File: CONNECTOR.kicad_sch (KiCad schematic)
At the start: 12 parts, among them J10 SWD, J17 SW_UART, J2 STM_IO, J7 CONNECTOR

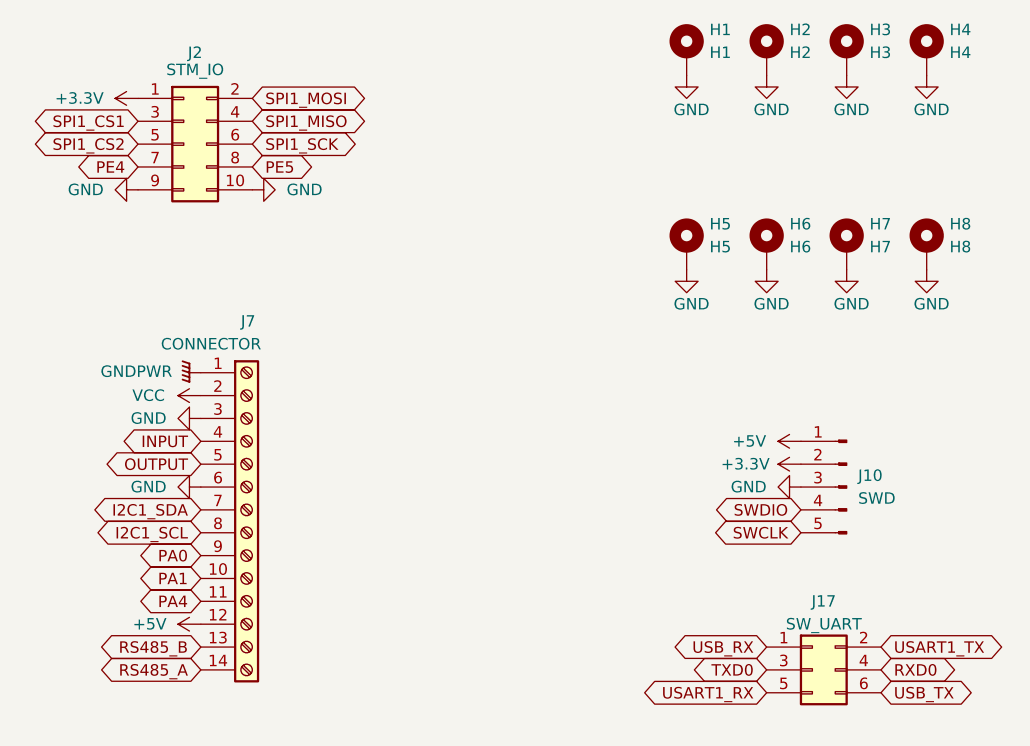
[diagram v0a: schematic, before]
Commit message: Add files via upload
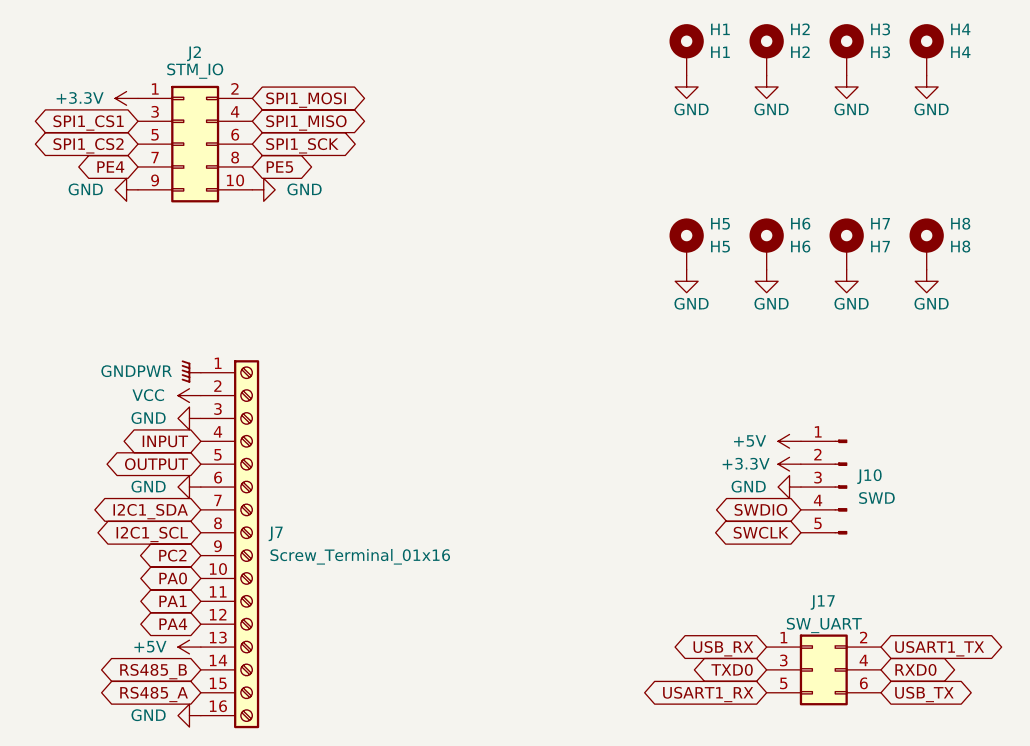
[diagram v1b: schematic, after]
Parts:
- removed J7: CONNECTOR, TerminalBlock_Phoenix:TerminalBlock_Phoenix_MKDS-1,5-14-5.08_1x14_P5.08mm_Horizontal, symbol Connector:Screw_Terminal_01x14
- added J7: Screw_Terminal_01x16, TerminalBlock_Phoenix:TerminalBlock_Phoenix_MKDS-1,5-16-5.08_1x16_P5.08mm_Horizontal, symbol Connector:Screw_Terminal_01x16
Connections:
- net +5V: now also J7.13 (Pin_13)
- net GND: now also J7.16 (Pin_16), J7.3 (Pin_3), J7.6 (Pin_6)
- net GNDPWR: now also J7.1 (Pin_1)
- net I2C1_SCL: now also J7.8 (Pin_8)
- net I2C1_SDA: now also J7.7 (Pin_7)
- net INPUT: now also J7.4 (Pin_4)
- net OUTPUT: now also J7.5 (Pin_5)
- net PA0: now also J7.10 (Pin_10)
- net PA1: now also J7.11 (Pin_11)
- net PA4: now also J7.12 (Pin_12)
- net RS485_A: now also J7.15 (Pin_15)
- net RS485_B: now also J7.14 (Pin_14)
- net VCC: now also J7.2 (Pin_2)
- new net PC2: J7.9 (Pin_9)
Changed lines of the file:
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@@
     )
   )
-  (global_label "RS485_A" (shape bidirectional) (at 71.12 93.345 180) (fields_autoplaced)
-    (effects (font (size 1.27 1.27)) (justify right))
-    (property "Intersheet References" "${INTERSHEET_REFS}" (id 0) (at 60.5426 93.4244 0)
+  (global_label "RS485_A" (shape bidirectional) (at 71.12 95.885 180) (fields_autoplaced)
+    (effects (font (size 1.27 1.27)) (justify right))
+    (property "Intersheet References" "${INTERSHEET_REFS}" (id 0) (at 60.5426 95.9644 0)
       (effects (font (size 1.27 1.27)) (justify right) hide)
     )
@@
     )
   )
-  (global_label "PA1" (shape bidirectional) (at 71.12 83.185 180) (fields_autoplaced)
+  (global_label "PA1" (shape bidirectional) (at 71.12 85.725 180) (fields_autoplaced)
+    (effects (font (size 1.27 1.27)) (justify right))
+    (property "Intersheet References" "${INTERSHEET_REFS}" (id 0) (at 65.1388 85.6456 0)
+      (effects (font (size 1.27 1.27)) (justify right) hide)
+    )
+  )
+  (global_label "INPUT" (shape bidirectional) (at 71.12 67.945 180) (fields_autoplaced)
+    (effects (font (size 1.27 1.27)) (justify right))
+    (property "Intersheet References" "${INTERSHEET_REFS}" (id 0) (at 63.2036 67.8656 0)
+      (effects (font (size 1.27 1.27)) (justify right) hide)
+    )
+  )
+  (global_label "I2C1_SDA" (shape bidirectional) (at 71.12 75.565 180) (fields_autoplaced)
+    (effects (font (size 1.27 1.27)) (justify right))
+    (property "Intersheet References" "${INTERSHEET_REFS}" (id 0) (at 59.8774 75.6444 0)
+      (effects (font (size 1.27 1.27)) (justify right) hide)
+    )
+  )
+  (global_label "PA4" (shape bidirectional) (at 71.12 88.265 180) (fields_autoplaced)
+    (effects (font (size 1.27 1.27)) (justify right))
+    (property "Intersheet References" "${INTERSHEET_REFS}" (id 0) (at 65.1388 88.1856 0)
+      (effects (font (size 1.27 1.27)) (justify right) hide)
+    )
+  )
+  (global_label "PA0" (shape bidirectional) (at 71.12 83.185 180) (fields_autoplaced)
     (effects (font (size 1.27 1.27)) (justify right))
     (property "Intersheet References" "${INTERSHEET_REFS}" (id 0) (at 65.1388 83.1056 0)
@@
     )
   )
-  (global_label "INPUT" (shape bidirectional) (at 71.12 67.945 180) (fields_autoplaced)
-    (effects (font (size 1.27 1.27)) (justify right))
-    (property "Intersheet References" "${INTERSHEET_REFS}" (id 0) (at 63.2036 67.8656 0)
-      (effects (font (size 1.27 1.27)) (justify right) hide)
-    )
-  )
-  (global_label "I2C1_SDA" (shape bidirectional) (at 71.12 75.565 180) (fields_autoplaced)
-    (effects (font (size 1.27 1.27)) (justify right))
-    (property "Intersheet References" "${INTERSHEET_REFS}" (id 0) (at 59.8774 75.6444 0)
-      (effects (font (size 1.27 1.27)) (justify right) hide)
-    )
-  )
-  (global_label "PA4" (shape bidirectional) (at 71.12 85.725 180) (fields_autoplaced)
-    (effects (font (size 1.27 1.27)) (justify right))
-    (property "Intersheet References" "${INTERSHEET_REFS}" (id 0) (at 65.1388 85.6456 0)
-      (effects (font (size 1.27 1.27)) (justify right) hide)
-    )
-  )
-  (global_label "PA0" (shape bidirectional) (at 71.12 80.645 180) (fields_autoplaced)
-    (effects (font (size 1.27 1.27)) (justify right))
-    (property "Intersheet References" "${INTERSHEET_REFS}" (id 0) (at 65.1388 80.5656 0)
-      (effects (font (size 1.27 1.27)) (justify right) hide)
-    )
-  )
   (global_label "SWCLK" (shape bidirectional) (at 137.795 78.105 180) (fields_autoplaced)
     (effects (font (size 1.27 1.27)) (justify right))
@@
     )
   )
-  (global_label "RS485_B" (shape bidirectional) (at 71.12 90.805 180) (fields_autoplaced)
-    (effects (font (size 1.27 1.27)) (justify right))
-    (property "Intersheet References" "${INTERSHEET_REFS}" (id 0) (at 60.3612 90.8844 0)
+  (global_label "RS485_B" (shape bidirectional) (at 71.12 93.345 180) (fields_autoplaced)
+    (effects (font (size 1.27 1.27)) (justify right))
+    (property "Intersheet References" "${INTERSHEET_REFS}" (id 0) (at 60.3612 93.4244 0)
+      (effects (font (size 1.27 1.27)) (justify right) hide)
+    )
+  )
+  (global_label "PC2" (shape bidirectional) (at 71.12 80.645 180) (fields_autoplaced)
+    (effects (font (size 1.27 1.27)) (justify right))
+    (property "Intersheet References" "${INTERSHEET_REFS}" (id 0) (at 64.9574 80.5656 0)
       (effects (font (size 1.27 1.27)) (justify right) hide)
     )
@@
     )
     (pin "1")
+  )
+  (symbol (lib_id "Connector:Screw_Terminal_01x16") (at 76.2 78.105 0) (unit 1)
+    (in_bom yes) (on_board yes) (fields_autoplaced)
+    (property "Reference" "J7" (id 0) (at 78.74 78.1049 0)
+      (effects (font (size 1.27 1.27)) (justify left))
+    )
+    (property "Value" "Screw_Terminal_01x16" (id 1) (at 78.74 80.6449 0)
+      (effects (font (size 1.27 1.27)) (justify left))
+    )
+    (property "Footprint" "TerminalBlock_Phoenix:TerminalBlock_Phoenix_MKDS-1,5-16-5.08_1x16_P5.08mm_Horizontal" (id 2) (at 76.2 78.105 0)
+      (effects (font (size 1.27 1.27)) hide)
+    )
+    (property "Datasheet" "~" (id 3) (at 76.2 78.105 0)
+      (effects (font (size 1.27 1.27)) hide)
+    )
+    (pin "1")
+    (pin "10")
+    (pin "11")
+    (pin "12")
+    (pin "13")
+    (pin "14")
+    (pin "15")
+    (pin "16")
+    (pin "2")
+    (pin "3")
+    (pin "4")
+    (pin "5")
+    (pin "6")
+    (pin "7")
+    (pin "8")
+    (pin "9")
   )
   (symbol (lib_id "power:GND") (at 133.985 48.895 0) (unit 1)
@@
     (pin "1")
   )
-  (symbol (lib_id "power:+5V") (at 71.12 88.265 90) (unit 1)
-    (in_bom yes) (on_board yes) (fields_autoplaced)
-    (property "Reference" "#PWR0162" (id 0) (at 74.93 88.265 0)
-      (effects (font (size 1.27 1.27)) hide)
-    )
-    (property "Value" "+5V" (id 1) (at 67.31 88.2649 90)
-      (effects (font (size 1.27 1.27)) (justify left))
-    )
-    (property "Footprint" "" (id 2) (at 71.12 88.265 0)
-      (effects (font (size 1.27 1.27)) hide)
-    )
-    (property "Datasheet" "" (id 3) (at 71.12 88.265 0)
-      (effects (font (size 1.27 1.27)) hide)
-    )
-    (pin "1")
-  )
-  (symbol (lib_id "Connector:Screw_Terminal_01x14") (at 76.2 75.565 0) (unit 1)
-    (in_bom yes) (on_board yes)
-    (property "Reference" "J7" (id 0) (at 75.565 54.61 0)
-      (effects (font (size 1.27 1.27)) (justify left))
-    )
-    (property "Value" "CONNECTOR" (id 1) (at 66.675 57.15 0)
-      (effects (font (size 1.27 1.27)) (justify left))
-    )
-    (property "Footprint" "TerminalBlock_Phoenix:TerminalBlock_Phoenix_MKDS-1,5-14-5.08_1x14_P5.08mm_Horizontal" (id 2) (at 76.2 75.565 0)
-      (effects (font (size 1.27 1.27)) hide)
-    )
-    (property "Datasheet" "~" (id 3) (at 76.2 75.565 0)
-      (effects (font (size 1.27 1.27)) hide)
-    )
-    (pin "1")
-    (pin "10")
-    (pin "11")
-    (pin "12")
-    (pin "13")
-    (pin "14")
-    (pin "2")
-    (pin "3")
-    (pin "4")
-    (pin "5")
-    (pin "6")
-    (pin "7")
-    (pin "8")
-    (pin "9")
+  (symbol (lib_id "power:+5V") (at 71.12 90.805 90) (unit 1)
+    (in_bom yes) (on_board yes) (fields_autoplaced)
+    (property "Reference" "#PWR0162" (id 0) (at 74.93 90.805 0)
+      (effects (font (size 1.27 1.27)) hide)
+    )
+    (property "Value" "+5V" (id 1) (at 67.31 90.8049 90)
+      (effects (font (size 1.27 1.27)) (justify left))
+    )
+    (property "Footprint" "" (id 2) (at 71.12 90.805 0)
+      (effects (font (size 1.27 1.27)) hide)
+    )
+    (property "Datasheet" "" (id 3) (at 71.12 90.805 0)
+      (effects (font (size 1.27 1.27)) hide)
+    )
+    (pin "1")
+  )
+  (symbol (lib_id "power:GND") (at 71.12 98.425 270) (unit 1)
+    (in_bom yes) (on_board yes)
+    (property "Reference" "#PWR0165" (id 0) (at 64.77 98.425 0)
+      (effects (font (size 1.27 1.27)) hide)
+    )
+    (property "Value" "GND" (id 1) (at 67.31 98.425 90)
+      (effects (font (size 1.27 1.27)) (justify right))
+    )
+    (property "Footprint" "" (id 2) (at 71.12 98.425 0)
+      (effects (font (size 1.27 1.27)) hide)
+    )
+    (property "Datasheet" "" (id 3) (at 71.12 98.425 0)
+      (effects (font (size 1.27 1.27)) hide)
+    )
+    (pin "1")
   )
   (symbol (lib_id "power:GNDPWR") (at 71.12 60.325 270) (unit 1)

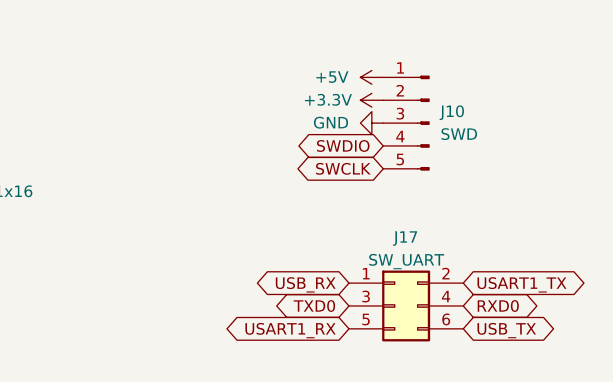
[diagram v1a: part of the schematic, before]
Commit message: Add files via upload
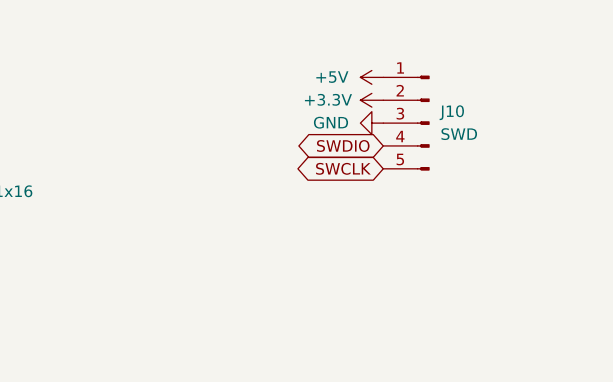
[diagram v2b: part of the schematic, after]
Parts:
- removed J17: SW_UART, Connector_PinHeader_2.54mm:PinHeader_2x03_P2.54mm_Vertical, symbol Connector_Generic:Conn_02x03_Odd_Even
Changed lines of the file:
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@@
-    )
-  )
-  (global_label "RXD0" (shape bidirectional) (at 146.685 93.345 0) (fields_autoplaced)
-    (effects (font (size 1.27 1.27)) (justify left))
-    (property "Intersheet References" "${INTERSHEET_REFS}" (id 0) (at 154.0571 93.2656 0)
-      (effects (font (size 1.27 1.27)) (justify left) hide)
     )
   )
@@
     )
   )
-  (global_label "TXD0" (shape bidirectional) (at 133.985 93.345 180) (fields_autoplaced)
-    (effects (font (size 1.27 1.27)) (justify right))
-    (property "Intersheet References" "${INTERSHEET_REFS}" (id 0) (at 126.9152 93.2656 0)
-      (effects (font (size 1.27 1.27)) (justify right) hide)
-    )
-  )
-  (global_label "USART1_TX" (shape bidirectional) (at 146.685 90.805 0) (fields_autoplaced)
-    (effects (font (size 1.27 1.27)) (justify left))
-    (property "Intersheet References" "${INTERSHEET_REFS}" (id 0) (at 159.3186 90.7256 0)
-      (effects (font (size 1.27 1.27)) (justify left) hide)
-    )
-  )
   (global_label "PE5" (shape bidirectional) (at 76.835 37.465 0) (fields_autoplaced)
     (effects (font (size 1.27 1.27)) (justify left))
@@
     )
   )
-  (global_label "USART1_RX" (shape bidirectional) (at 133.985 95.885 180) (fields_autoplaced)
-    (effects (font (size 1.27 1.27)) (justify right))
-    (property "Intersheet References" "${INTERSHEET_REFS}" (id 0) (at 121.049 95.8056 0)
-      (effects (font (size 1.27 1.27)) (justify right) hide)
-    )
-  )
   (global_label "RS485_A" (shape bidirectional) (at 71.12 95.885 180) (fields_autoplaced)
     (effects (font (size 1.27 1.27)) (justify right))
     (property "Intersheet References" "${INTERSHEET_REFS}" (id 0) (at 60.5426 95.9644 0)
-      (effects (font (size 1.27 1.27)) (justify right) hide)
-    )
-  )
-  (global_label "USB_RX" (shape bidirectional) (at 133.985 90.805 180) (fields_autoplaced)
-    (effects (font (size 1.27 1.27)) (justify right))
-    (property "Intersheet References" "${INTERSHEET_REFS}" (id 0) (at 124.3148 90.8844 0)
       (effects (font (size 1.27 1.27)) (justify right) hide)
     )
@@
     (effects (font (size 1.27 1.27)) (justify left))
     (property "Intersheet References" "${INTERSHEET_REFS}" (id 0) (at 89.1057 32.3056 0)
-      (effects (font (size 1.27 1.27)) (justify left) hide)
-    )
-  )
-  (global_label "USB_TX" (shape bidirectional) (at 146.685 95.885 0) (fields_autoplaced)
-    (effects (font (size 1.27 1.27)) (justify left))
-    (property "Intersheet References" "${INTERSHEET_REFS}" (id 0) (at 156.0529 95.8056 0)
       (effects (font (size 1.27 1.27)) (justify left) hide)
     )
@@
     (pin "1")
   )
-  (symbol (lib_id "Connector_Generic:Conn_02x03_Odd_Even") (at 139.065 93.345 0) (unit 1)
-    (in_bom yes) (on_board yes)
-    (property "Reference" "J17" (id 0) (at 140.335 85.725 0))
-    (property "Value" "SW_UART" (id 1) (at 140.335 88.265 0))
-    (property "Footprint" "Connector_PinHeader_2.54mm:PinHeader_2x03_P2.54mm_Vertical" (id 2) (at 139.065 93.345 0)
-      (effects (font (size 1.27 1.27)) hide)
-    )
-    (property "Datasheet" "~" (id 3) (at 139.065 93.345 0)
-      (effects (font (size 1.27 1.27)) hide)
-    )
-    (pin "1")
-    (pin "2")
-    (pin "3")
-    (pin "4")
-    (pin "5")
-    (pin "6")
-  )
   (symbol (lib_id "power:GND") (at 137.795 73.025 270) (unit 1)
